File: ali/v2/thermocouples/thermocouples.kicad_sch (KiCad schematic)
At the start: 4 parts

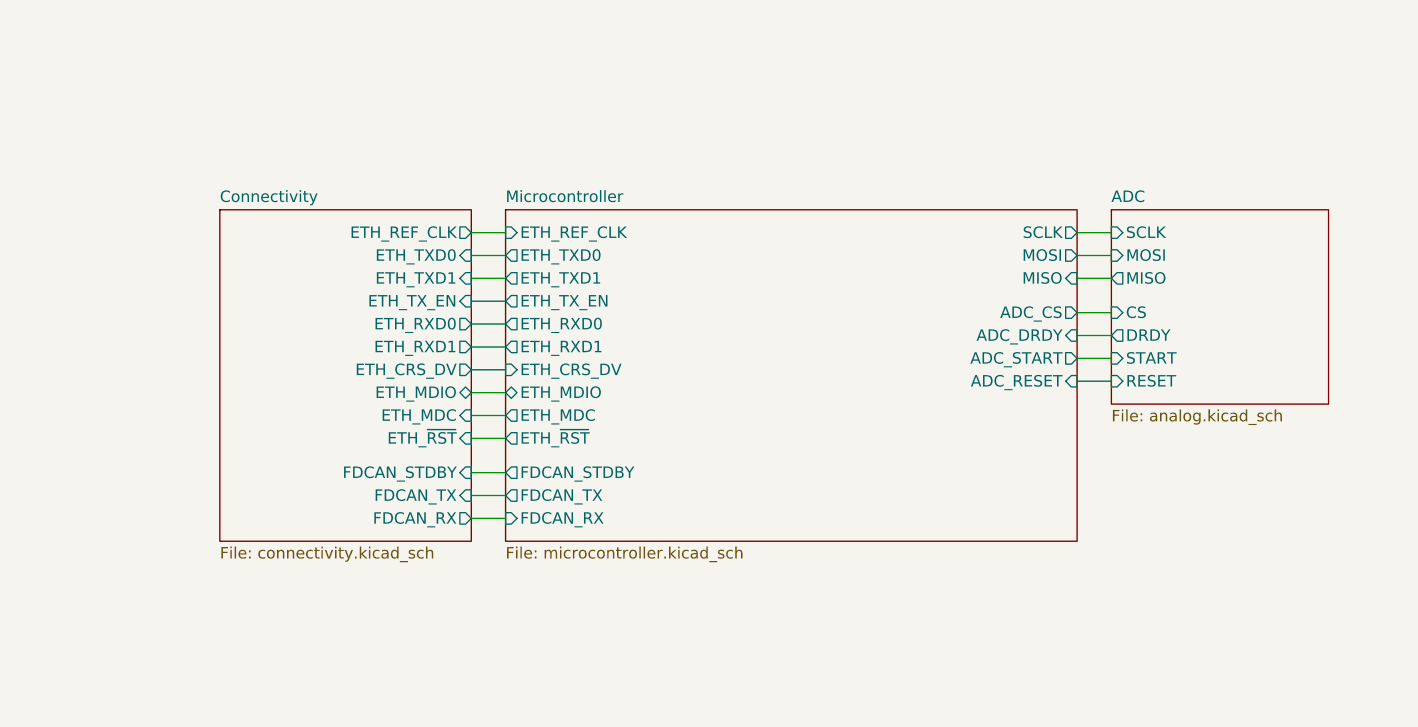
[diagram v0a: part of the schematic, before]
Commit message: mfw tcs
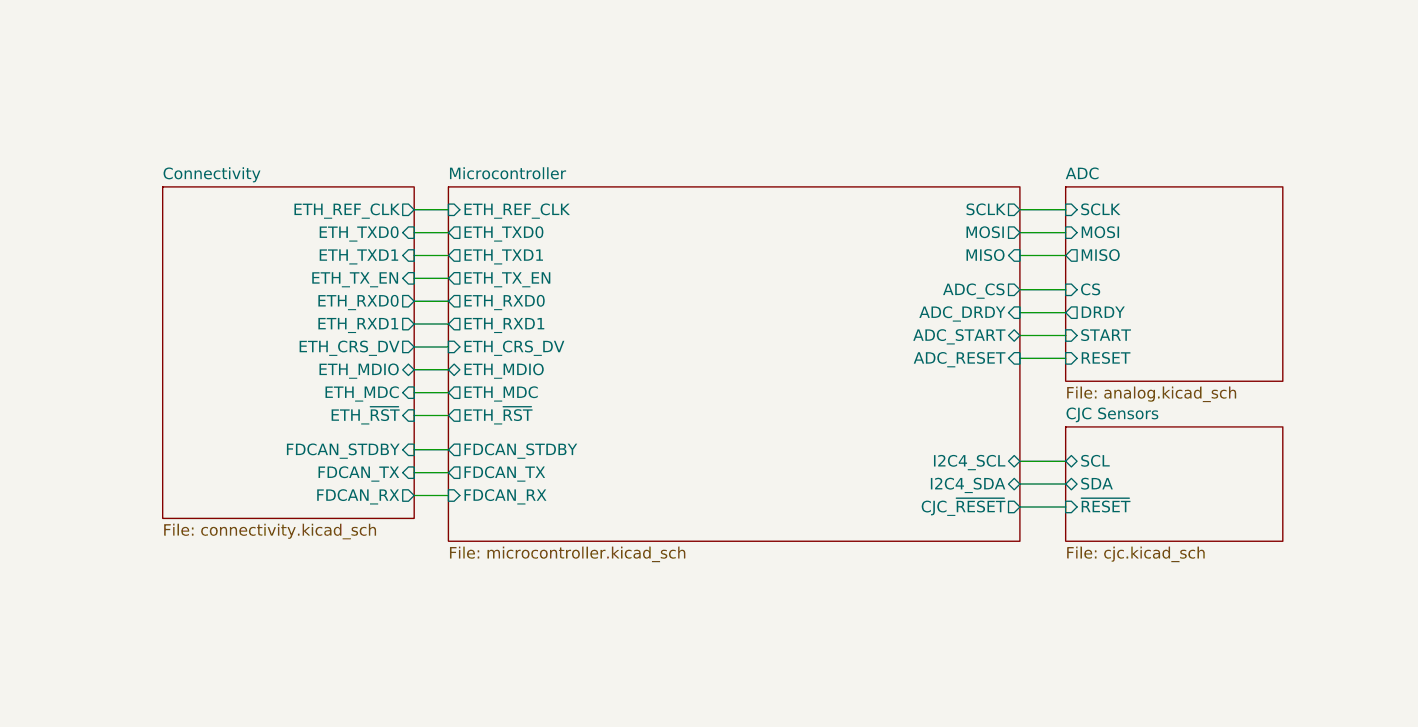
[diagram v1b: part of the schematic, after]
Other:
- added sheet CJC Sensors (cjc.kicad_sch)
- sheet Microcontroller ports: added CJC_~{RESET}, I2C4_SCL, I2C4_SDA; removed none
